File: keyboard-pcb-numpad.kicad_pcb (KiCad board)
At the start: 2 copper layers, 100 x 99 mm, 37 parts, among them SW1 SW_Push, U1 ProMicro

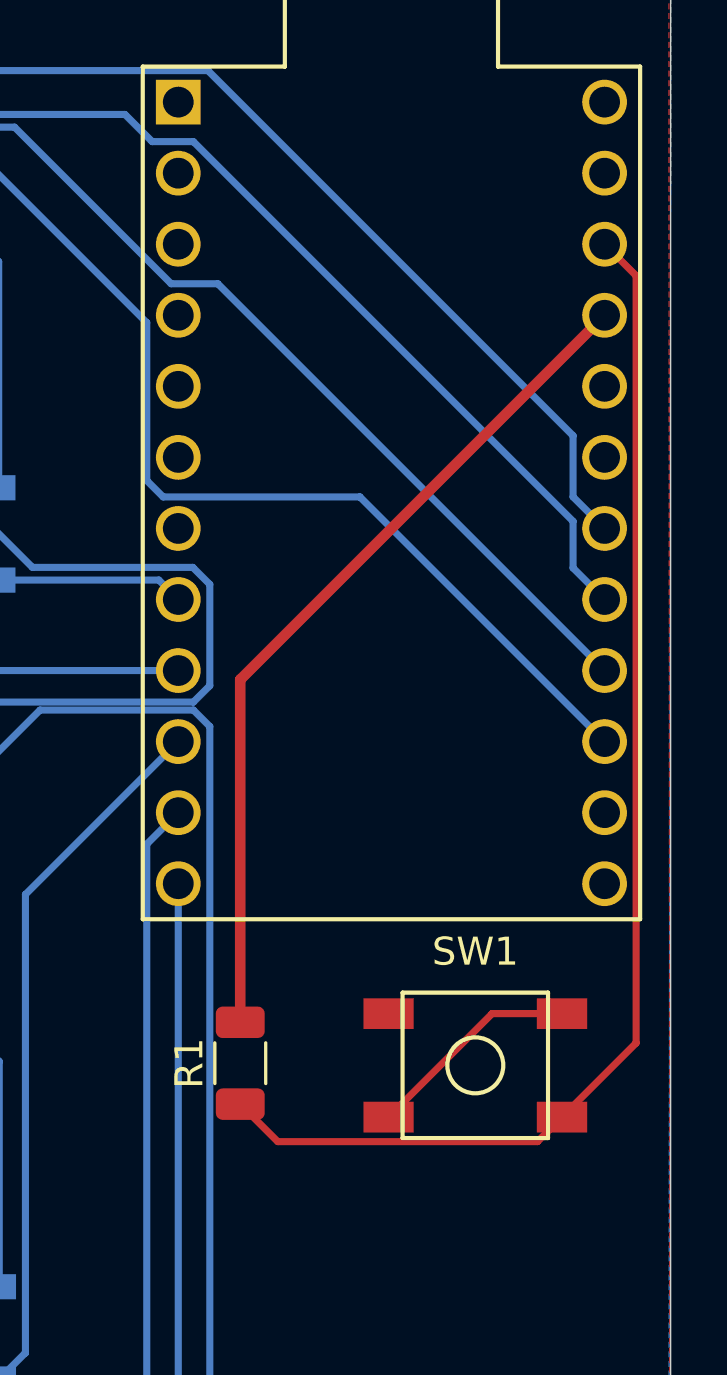
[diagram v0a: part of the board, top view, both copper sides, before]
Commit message: fix: fix pcb
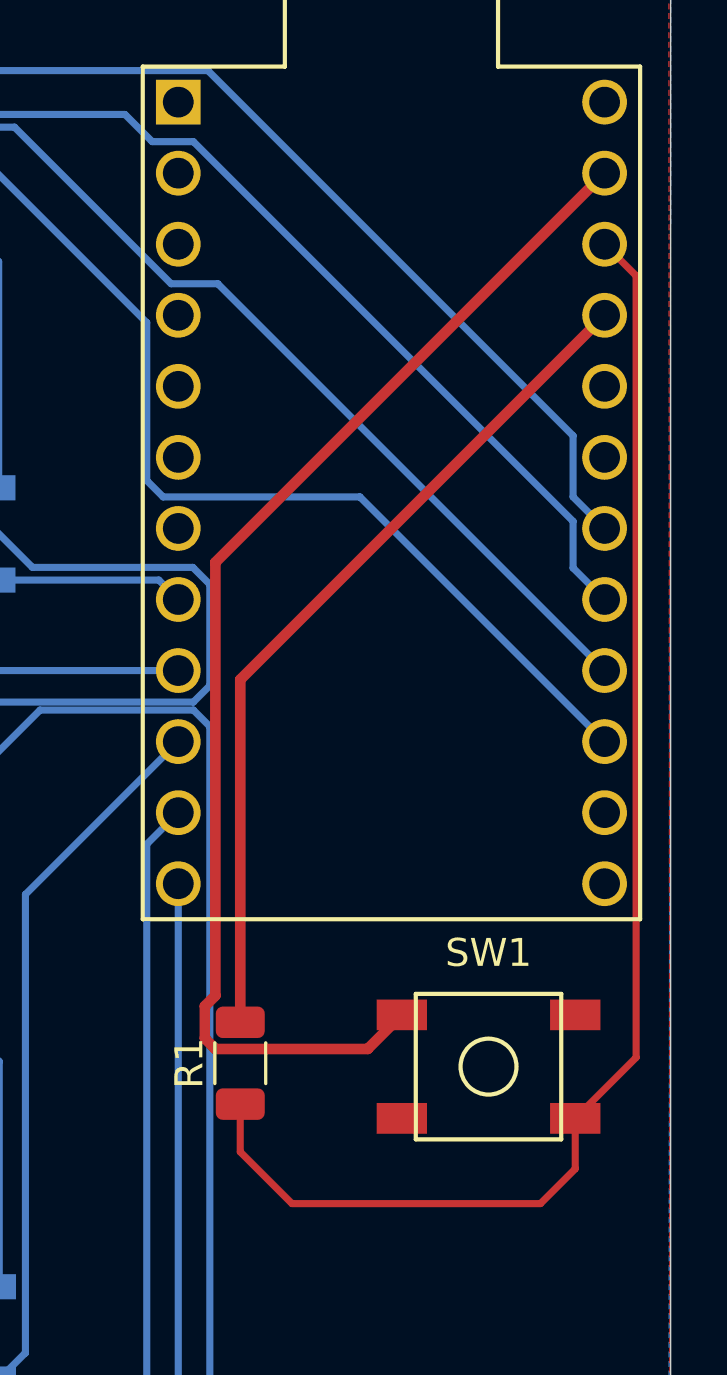
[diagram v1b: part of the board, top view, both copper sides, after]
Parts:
- moved SW1 0.47 mm to (131.5, 81.5)
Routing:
- net GND: track 0.00 -> 44.6 mm
- net (no net): track 7.73 -> 0.00 mm
- net /RST: track 45.2 -> 49.4 mm
